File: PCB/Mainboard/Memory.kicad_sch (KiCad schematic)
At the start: 29 parts, among them J15 RAM Module, U28 M5M4V16160, U33 M5M4V16160

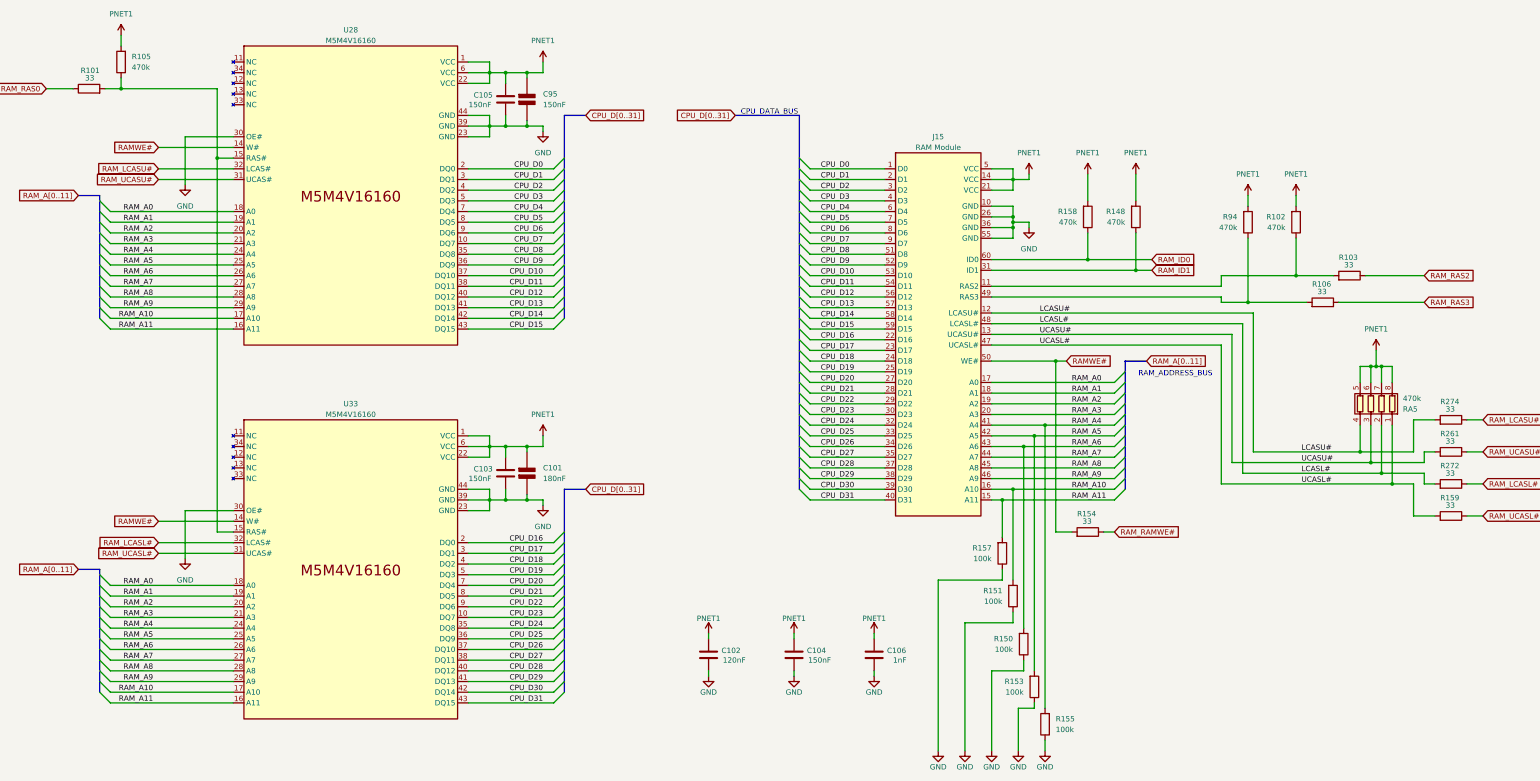
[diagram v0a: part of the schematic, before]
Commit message: Add files via upload
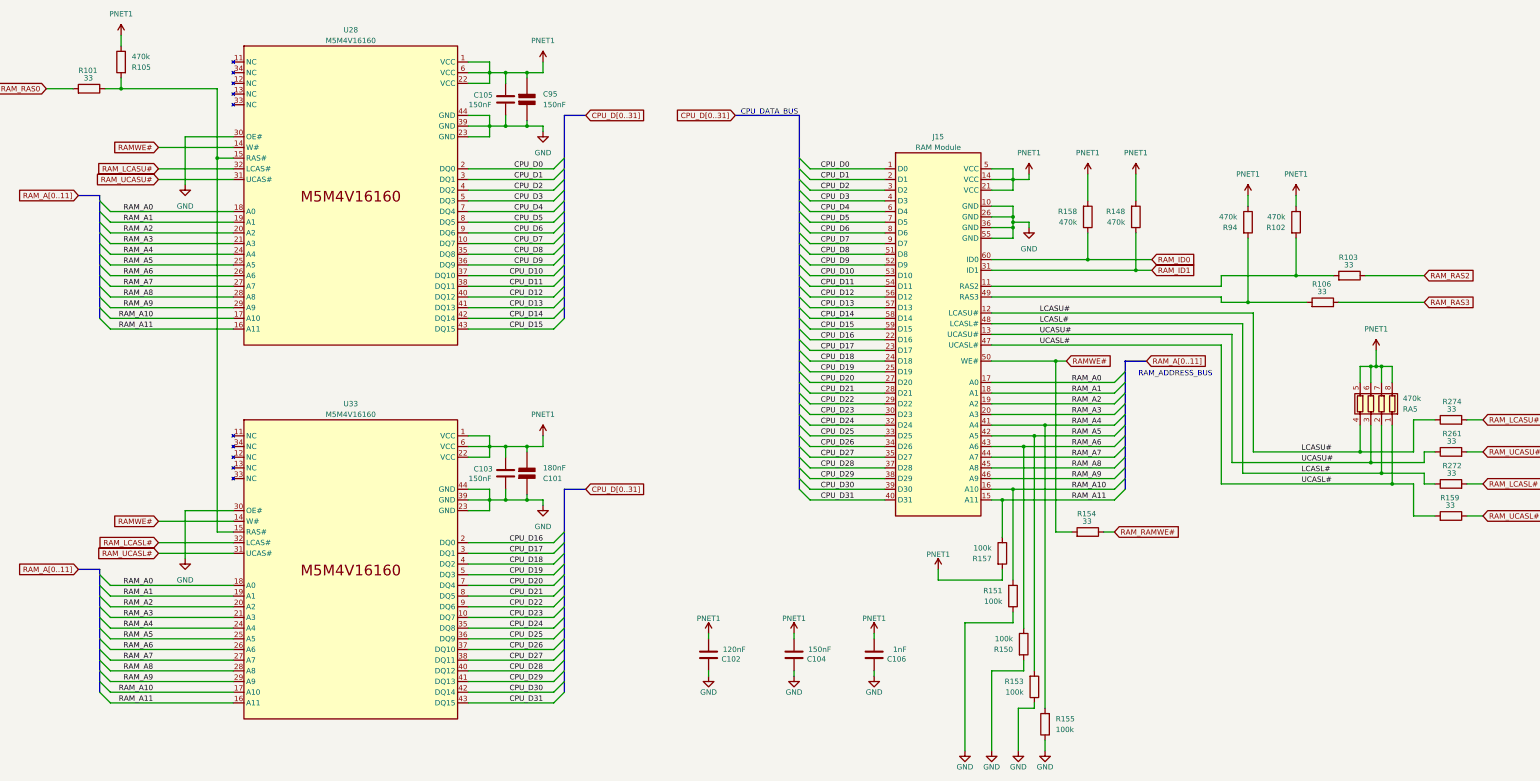
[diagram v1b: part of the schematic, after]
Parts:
- C101, C102, C103, C104, C105, C106, C95: footprint (none) -> Capacitor_SMD:C_0402_1005Metric
- J15: footprint (none) -> PC110:RAM Module
- R101, R102, R103, R105, R106, R148, R150, R151, R153, R154, R155, R157, R158, R159, R261, R272, R274, R94: footprint (none) -> PCM_Resistor_SMD_AKL:R_0402_1005Metric
- RA5: footprint (none) -> PC110:R-array
- U28, U33: footprint (none) -> PC110:RAMchip
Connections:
- net GND: now also C101.1 (+), C102.1, C104.1, C106.1, R150.2; no longer C101.2 (-), C102.2, C104.2, C106.2, R150.1, R157.1
- net LCASL#: now also R272.1; no longer R272.2
- net LCASU#: now also R274.1; no longer R274.2
- net PNET1: now also C101.2 (-), C102.2, C104.2, C106.2, R102.1, R105.1, R157.2, R94.1; no longer C101.1 (+), C102.1, C104.1, C106.1, R102.2, R105.2, R94.2
- net RAM_A11: now also R157.1; no longer R157.2
- net RAM_A6: now also R150.1; no longer R150.2
- net RAM_LCASL#: now also R272.2; no longer R272.1
- net RAM_LCASU#: now also R274.2; no longer R274.1
- net RAM_RAS0: now also R101.2; no longer R101.1
- net RAM_UCASU#: now also R261.2; no longer R261.1
- net UCASU#: now also R261.1; no longer R261.2
- net at J15.11 (RAS2), R103.2: now also R102.2; no longer R102.1
- net at J15.49 (RAS3), R106.2: now also R94.2; no longer R94.1
- net at U28.15 (RAS#), U33.15 (RAS#): now also R101.1, R105.2; no longer R101.2, R105.1
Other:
- moved on the sheet: C102, C104, C106, R101, R105, R261, R272, R274

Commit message: Add files via upload
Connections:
- net LCASL#: now also R272.2; no longer R272.1
- net LCASU#: now also R274.2; no longer R274.1
- net UCASL#: now also R159.1; no longer R159.2
- net UCASU#: now also R261.2; no longer R261.1
- net RAM_LCASL# renamed U61_RAM_LCASL#
- net U61_RAM_LCASL#: now also R272.1; no longer R272.2
- net RAM_LCASU# renamed U61_RAM_LCASU#
- net U61_RAM_LCASU#: now also R274.1; no longer R274.2
- net RAM_RAMWE# renamed U61_RAM_RAMWE#
- net RAM_RAS0 renamed U61_RAM_RAS0
- net RAM_RAS2 renamed U61_RAM_RAS2
- net RAM_RAS3 renamed U61_RAM_RAS3
- net RAM_UCASL# renamed U61_RAM_UCASL#
- net U61_RAM_UCASL#: now also R159.2; no longer R159.1
- net RAM_UCASU# renamed U61_RAM_UCASU#
- net U61_RAM_UCASU#: now also R261.1; no longer R261.2
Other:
- moved on the sheet: R159, R261, R272, R274
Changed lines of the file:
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@@
 		)
 	)
-	(global_label "RAM_LCASU#"
+	(global_label "U61_RAM_LCASU#"
 		(shape input)
 		(at 66.04 93.98 180)
@@
 		)
 		(property "Intersheetrefs" "${INTERSHEET_REFS}"
-			(at 51.0805 93.98 0)
+			(at 46.3634 93.98 0)
 			(effects
 				(font
@@
 		)
 	)
-	(global_label "RAM_RAMWE#"
+	(global_label "U61_RAM_RAMWE#"
 		(shape input)
 		(at 293.37 180.34 0)
@@
 		)
 		(property "Intersheetrefs" "${INTERSHEET_REFS}"
-			(at 308.8132 180.34 0)
+			(at 313.5303 180.34 0)
 			(effects
 				(font
@@
 		)
 	)
-	(global_label "RAM_UCASL#"
+	(global_label "U61_RAM_UCASL#"
 		(shape input)
 		(at 381 176.53 0)
@@
 		)
 		(property "Intersheetrefs" "${INTERSHEET_REFS}"
-			(at 395.9595 176.53 0)
+			(at 400.6766 176.53 0)
 			(effects
 				(font
@@
 		)
 	)
-	(global_label "RAM_LCASU#"
+	(global_label "U61_RAM_LCASU#"
 		(shape input)
 		(at 381 153.67 0)
@@
 		)
 		(property "Intersheetrefs" "${INTERSHEET_REFS}"
-			(at 395.9595 153.67 0)
+			(at 400.6766 153.67 0)
 			(effects
 				(font
@@
 		)
 	)
-	(global_label "RAM_UCASL#"
+	(global_label "U61_RAM_UCASL#"
 		(shape input)
 		(at 66.04 185.42 180)
@@
 		)
 		(property "Intersheetrefs" "${INTERSHEET_REFS}"
-			(at 51.0805 185.42 0)
+			(at 46.3634 185.42 0)
 			(effects
 				(font
@@
 		)
 	)
-	(global_label "RAM_RAS2"
+	(global_label "U61_RAM_RAS2"
 		(shape input)
 		(at 367.03 119.38 0)
@@
 		)
 		(property "Intersheetrefs" "${INTERSHEET_REFS}"
-			(at 379.5704 119.38 0)
+			(at 384.2875 119.38 0)
 			(effects
 				(font
@@
 		)
 	)
-	(global_label "RAM_RAS0"
+	(global_label "U61_RAM_RAS0"
 		(shape input)
 		(at 39.37 74.93 180)
@@
 		)
 		(property "Intersheetrefs" "${INTERSHEET_REFS}"
-			(at 26.8296 74.93 0)
+			(at 22.1125 74.93 0)
 			(effects
 				(font
@@
 		)
 	)
-	(global_label "RAM_UCASU#"
+	(global_label "U61_RAM_UCASU#"
 		(shape input)
 		(at 381 161.29 0)
@@
 		)
 		(property "Intersheetrefs" "${INTERSHEET_REFS}"
-			(at 396.2619 161.29 0)
+			(at 400.979 161.29 0)
 			(effects
 				(font
@@
 		)
 	)
-	(global_label "RAM_LCASL#"
+	(global_label "U61_RAM_LCASL#"
 		(shape input)
 		(at 381 168.91 0)
@@
 		)
 		(property "Intersheetrefs" "${INTERSHEET_REFS}"
-			(at 395.6571 168.91 0)
+			(at 400.3742 168.91 0)
 			(effects
 				(font
@@
 		)
 	)
-	(global_label "RAM_RAS3"
+	(global_label "U61_RAM_RAS3"
 		(shape input)
 		(at 367.03 125.73 0)
@@
 		)
 		(property "Intersheetrefs" "${INTERSHEET_REFS}"
-			(at 379.5704 125.73 0)
+			(at 384.2875 125.73 0)
 			(effects
 				(font
@@
 		)
 	)
-	(global_label "RAM_LCASL#"
+	(global_label "U61_RAM_LCASL#"
 		(shape input)
 		(at 66.04 182.88 180)
@@
 		)
 		(property "Intersheetrefs" "${INTERSHEET_REFS}"
-			(at 51.3829 182.88 0)
+			(at 46.6658 182.88 0)
 			(effects
 				(font
@@
 		)
 	)
-	(global_label "RAM_UCASU#"
+	(global_label "U61_RAM_UCASU#"
 		(shape input)
 		(at 66.04 96.52 180)
@@
 		)
 		(property "Intersheetrefs" "${INTERSHEET_REFS}"
-			(at 50.7781 96.52 0)
+			(at 46.061 96.52 0)
 			(effects
 				(font
@@
 	(symbol
 		(lib_id "Device:R")
-		(at 373.38 161.29 90)
+		(at 373.38 161.29 270)
+		(mirror x)
 		(unit 1)
 		(exclude_from_sim no)
@@
 		(dnp no)
 		(property "Reference" "R261"
-			(at 375.92 156.972 90)
+			(at 370.84 156.972 90)
 			(effects
 				(font
@@
 		)
 		(property "Value" "33"
-			(at 374.6499 158.75 90)
+			(at 372.1101 158.75 90)
 			(effects
 				(font
@@
 	(symbol
 		(lib_id "Device:R")
-		(at 373.38 168.91 90)
+		(at 373.38 168.91 270)
+		(mirror x)
 		(unit 1)
 		(exclude_from_sim no)
@@
 		(dnp no)
 		(property "Reference" "R272"
-			(at 375.92 164.592 90)
+			(at 370.84 164.592 90)
 			(effects
 				(font
@@
 		)
 		(property "Value" "33"
-			(at 374.6499 166.37 90)
+			(at 372.1101 166.37 90)
 			(effects
 				(font
@@
 	(symbol
 		(lib_id "Device:R")
-		(at 373.38 176.53 270)
-		(mirror x)
+		(at 373.38 176.53 90)
 		(unit 1)
 		(exclude_from_sim no)
@@
 		(dnp no)
 		(property "Reference" "R159"
-			(at 370.84 172.212 90)
+			(at 375.92 172.212 90)
 			(effects
 				(font
@@
 		)
 		(property "Value" "33"
-			(at 372.1101 173.99 90)
+			(at 374.6499 173.99 90)
 			(effects
 				(font
@@
 	(symbol
 		(lib_id "Device:R")
-		(at 373.38 153.67 90)
+		(at 373.38 153.67 270)
+		(mirror x)
 		(unit 1)
 		(exclude_from_sim no)
@@
 		(dnp no)
 		(property "Reference" "R274"
-			(at 375.92 149.352 90)
+			(at 370.84 149.352 90)
 			(effects
 				(font
@@
 		)
 		(property "Value" "33"
-			(at 374.6499 151.13 90)
+			(at 372.1101 151.13 90)
 			(effects
 				(font

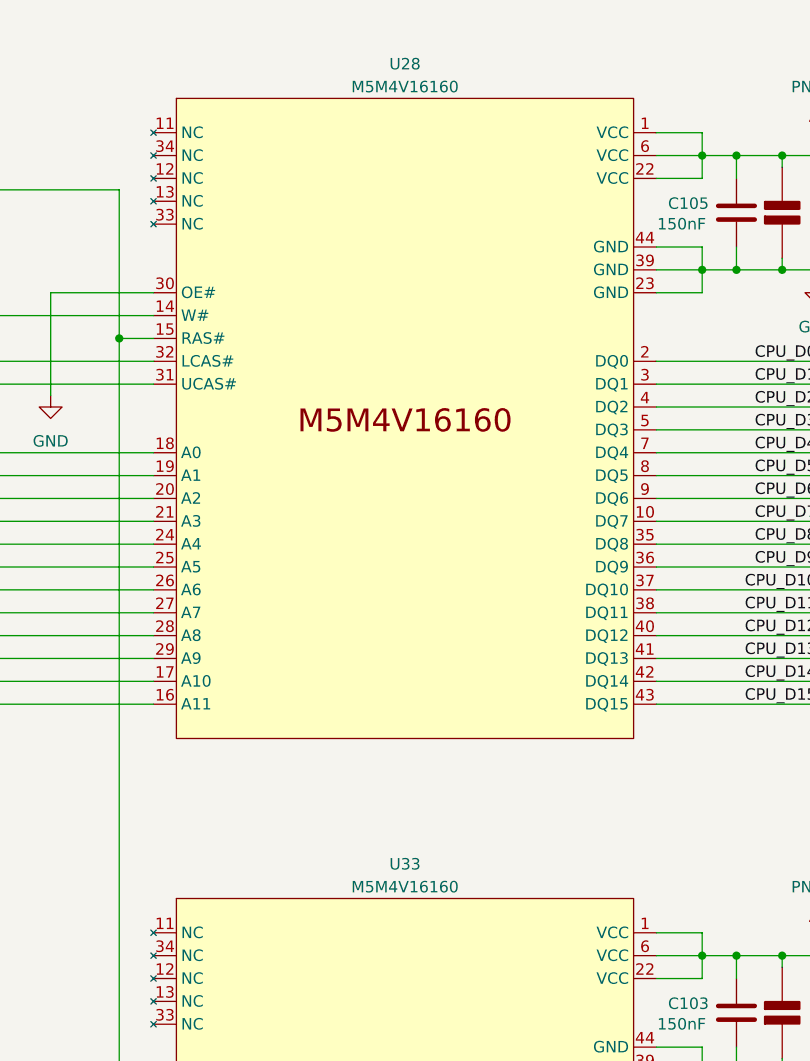
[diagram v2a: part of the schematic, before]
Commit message: Add files via upload
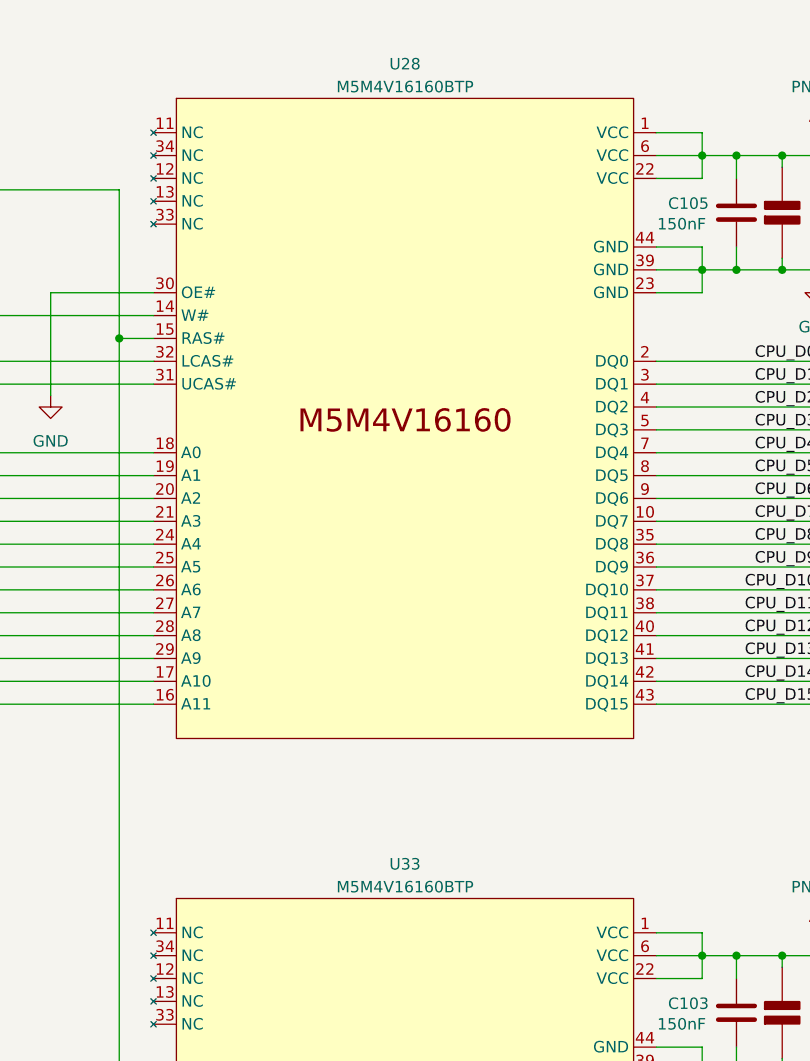
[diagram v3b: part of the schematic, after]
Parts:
- C101, C95: Indicator + -> (none); Rating V -> (none)
- U28, U33: value M5M4V16160 -> M5M4V16160BTP
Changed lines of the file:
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@@
 			)
 		)
-		(property "Description" "Resistor"
+		(property "Description" ""
 			(at 336.55 106.68 0)
 			(effects
@@
 			)
 		)
-		(property "Description" "Unpolarized capacitor"
+		(property "Description" ""
 			(at 148.59 166.37 0)
 			(effects
@@
 			)
 		)
-		(property "Description" "4 resistor network, parallel topology"
+		(property "Description" ""
 			(at 354.33 149.86 0)
 			(effects
@@
 			)
 		)
-		(property "Description" "Resistor"
+		(property "Description" ""
 			(at 298.45 105.41 0)
 			(effects
@@
 			)
 		)
-		(property "Description" "Resistor"
+		(property "Description" ""
 			(at 287.02 105.41 0)
 			(effects
@@
 			)
 		)
-		(property "Description" "Unpolarized capacitor"
+		(property "Description" ""
 			(at 196.85 209.55 0)
 			(effects
@@
 			)
 		)
-		(property "Description" "Resistor"
+		(property "Description" ""
 			(at 373.38 161.29 0)
 			(effects
@@
 			)
 		)
-		(property "Description" "Resistor"
+		(property "Description" ""
 			(at 266.7 185.42 0)
 			(effects
@@
 			)
 		)
-		(property "Description" "Resistor"
+		(property "Description" ""
 			(at 373.38 168.91 0)
 			(effects
@@
 			)
 		)
-		(property "Description" "Resistor"
+		(property "Description" ""
 			(at 342.9 125.73 0)
 			(effects
@@
 			)
 		)
-		(property "Description" "Resistor"
+		(property "Description" ""
 			(at 271.78 207.01 0)
 			(effects
@@
 			)
 		)
-		(property "Description" "Resistor"
+		(property "Description" ""
 			(at 57.15 68.58 0)
 			(effects
@@
 			)
 		)
-		(property "Description" "Resistor"
+		(property "Description" ""
 			(at 49.53 74.93 0)
 			(effects
@@
 			)
 		)
-		(property "Description" "Resistor"
+		(property "Description" ""
 			(at 349.25 119.38 0)
 			(effects
@@
 			)
 		)
-		(property "Value" "M5M4V16160"
+		(property "Value" "M5M4V16160BTP"
 			(at 111.76 152.4 0)
 			(effects
@@
 			)
 		)
-		(property "Description" "Resistor"
+		(property "Description" ""
 			(at 269.24 195.58 0)
 			(effects
@@
 			)
 		)
-		(property "Description" "Unpolarized capacitor"
+		(property "Description" ""
 			(at 148.59 77.47 0)
 			(effects
@@
 			)
 		)
-		(property "Description" "Unpolarized capacitor"
+		(property "Description" ""
 			(at 236.22 209.55 0)
 			(effects
@@
 			)
 		)
-		(property "Description" "Resistor"
+		(property "Description" ""
 			(at 373.38 176.53 0)
 			(effects
@@
 			)
 		)
-		(property "Value" "M5M4V16160"
+		(property "Value" "M5M4V16160BTP"
 			(at 111.76 63.5 0)
 			(effects
@@
 			)
 		)
-		(property "Description" "capacitor, non-polarized/bipolar"
+		(property "Description" ""
 			(at 153.67 166.37 0)
 			(effects
@@
 			)
 		)
-		(property "Indicator" "+"
-			(at 152.4 169.545 0)
-			(effects
-				(font
-					(size 1.27 1.27)
-				)
-				(hide yes)
-			)
-		)
-		(property "Rating" "V"
-			(at 153.035 163.195 0)
-			(effects
-				(font
-					(size 1.27 1.27)
-				)
-				(justify right)
-				(hide yes)
-			)
-		)
 		(pin "1"
 		)
@@
 			)
 		)
-		(property "Description" "capacitor, non-polarized/bipolar"
+		(property "Description" ""
 			(at 153.67 77.47 0)
 			(effects
@@
 			)
 		)
-		(property "Indicator" "+"
-			(at 152.4 74.295 0)
-			(effects
-				(font
-					(size 1.27 1.27)
-				)
-				(hide yes)
-			)
-		)
-		(property "Rating" "V"
-			(at 153.035 80.645 0)
-			(effects
-				(font
-					(size 1.27 1.27)
-				)
-				(justify right)
-				(hide yes)
-			)
-		)
 		(pin "1"
 		)
@@
 			)
 		)
-		(property "Description" "Resistor"
+		(property "Description" ""
 			(at 373.38 153.67 0)
 			(effects
@@
 			)
 		)
-		(property "Description" "Resistor"
+		(property "Description" ""
 			(at 287.02 180.34 0)
 			(effects
@@
 			)
 		)
-		(property "Description" "Unpolarized capacitor"
+		(property "Description" ""
 			(at 217.17 209.55 0)
 			(effects
@@
 			)
 		)
-		(property "Description" "Resistor"
+		(property "Description" ""
 			(at 274.32 217.17 0)
 			(effects
@@
 			)
 		)
-		(property "Description" "Resistor"
+		(property "Description" ""
 			(at 276.86 226.06 0)
 			(effects
@@
 			)
 		)
-		(property "Description" "Resistor"
+		(property "Description" ""
 			(at 325.12 106.68 0)
 			(effects
